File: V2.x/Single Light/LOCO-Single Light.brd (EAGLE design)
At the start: 25.1 x 16.5 mm, 32 parts, among them IC1 Atmega 328-P, IC2 MCP2515, IC3 MIC5219BM5, Q1 8MHz, Q2 16MHz

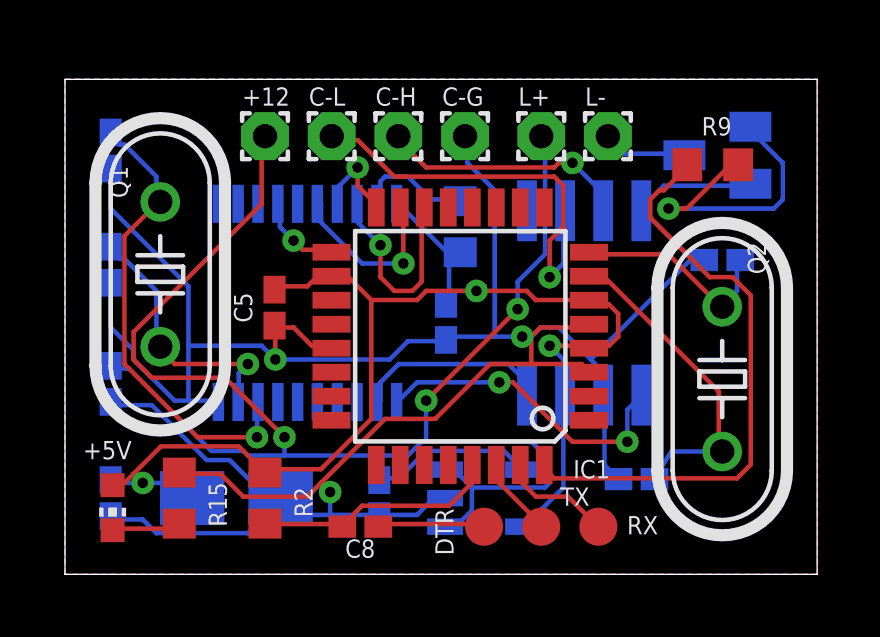
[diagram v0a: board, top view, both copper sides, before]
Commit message: initial
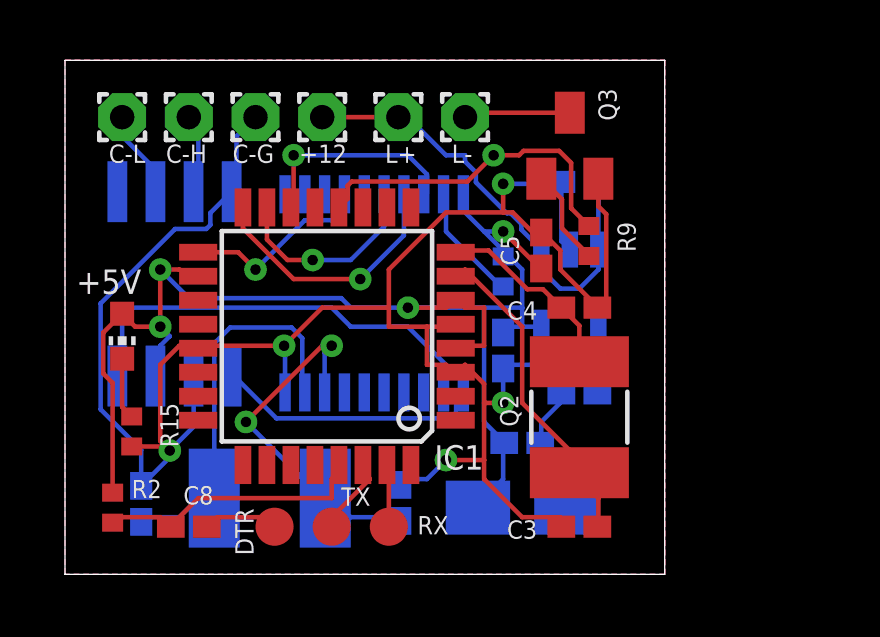
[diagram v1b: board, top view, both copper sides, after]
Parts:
- removed T1: (no value), transistor-neu-to92:SOT23-BEC
- added Q3: BSS123, transistor-small-signal:SOT23
- Q1, Q2: device crystal:HC49/S -> crystal-geyer_V1_0:5.0X3.2_2
- R1, R15, R2, R9: device rcl:R0603 -> rcl:R0402
- moved C11 17.0 mm to (17.1, 13.1), turned to 180 degrees
- moved C2 15.2 mm to (11.2, 2.38), turned to 90 degrees
- moved C15 13.8 mm to (15.2, 4.38), turned to 0 degrees
- moved DA1 13.7 mm to (3.65, 9.68)
- moved C16 9.53 mm to (15.2, 2.22)
- moved C5 9.09 mm to (15.9, 10.8), turned to 270 degrees
- moved Q1 8.31 mm to (6.83, 2.54), flipped to the bottom, turned to 180 degrees
- moved C1 8.03 mm to (2.54, 2.35), turned to 90 degrees
- moved IC3 7.55 mm to (16.8, 9.53), turned to 180 degrees
- moved C7 7.53 mm to (17.1, 6.03), turned to 180 degrees
- moved C-G 7.01 mm to (6.35, 15.2)
- moved C-H 7.01 mm to (4.13, 15.2)
- moved C-L 7.01 mm to (1.91, 15.2)
- moved RX 6.99 mm to (10.8, 1.59)
- moved DTR 6.99 mm to (6.99, 1.59)
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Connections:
- net D2: no longer R9.2
- net D8: now also R9.2
- net GND: now also Q3.2; no longer T1.E
- net LIGHT: now also Q3.3; no longer T1.C
- net N$2: now also Q3.1; no longer T1.B
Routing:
- net +12V: track 50.6 -> 15.6 mm, vias 3 -> 0
- net D2: track 19.7 -> 0.00 mm
- net GND: track 96.6 -> 79.8 mm, vias 3 -> 5
- net D8: track 0.00 -> 11.3 mm, vias 0 -> 1
- net CAN-L: track 14.1 -> 3.03 mm, vias 1 -> 0
- net RXCAN: track 6.55 -> 14.8 mm
- net N$2: track 9.75 -> 3.23 mm, vias 1 -> 0
- net SI: track 3.07 -> 8.74 mm
- net CAN-H: track 8.39 -> 2.82 mm, vias 1 -> 0
- net CAN-OCC1: track 8.75 -> 13.2 mm, vias 1 -> 0
- net SCK: track 2.92 -> 6.44 mm
- net N$1: track 5.46 -> 2.25 mm
- net CAN-OCC2: track 15.6 -> 12.6 mm, vias 1 -> 2
- net RX: track 3.75 -> 2.06 mm
- net VCC: track 46.5 -> 48.2 mm, vias 3 -> 4
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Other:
- board size 25.1 x 16.5 mm -> 20 x 17.1 mm

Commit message: initial
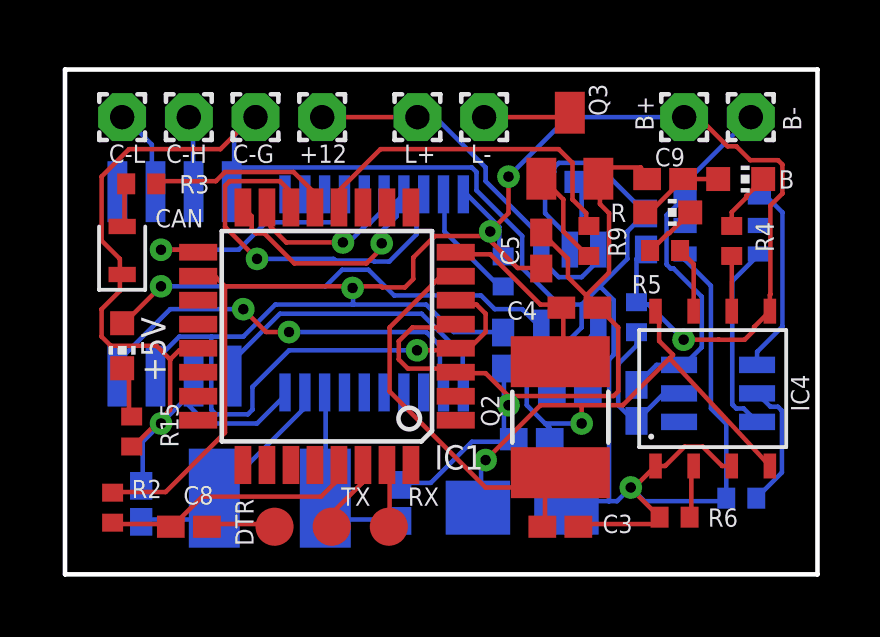
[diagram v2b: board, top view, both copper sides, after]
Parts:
- added B, R: (no value), led:CHIP-LED0603
- added B+, B-: (no value), wirepad:1,6/0,8
- added C10: 0,1µ, rcl:C0402K
- added C12: 10µ, rcl:C0402K
- added C9: 100n, rcl:C0402K
- added CAN: LED1, Opto-Electronic:LEDC1608X39N_B
- added IC4: TP4056, TP4056:SOT23-8
- added IC5: DW01A, DW01a:SOT23-6
- added Q4: FS8205ASOT-23-6L_TCP-L, FS8205A:SOT-23-6L_TCP-L
- added R3: 220R, rcl:R0402
- added R4, R5, R7: 1k, rcl:R0402
- added R6: 1k2, rcl:R0402
- added R8: 100R, rcl:R0402
- R15: value 10k -> 220R
- moved L+ 0.63 mm to (11.7, 15.2)
- moved L- 0.63 mm to (14.0, 15.2)
- moved C11 0.63 mm to (16.5, 13.1)
- moved C3 0.63 mm to (16.5, 1.59), turned to 0 degrees
- moved Q2 0.63 mm to (16.5, 5.24)
- moved C15 0.34 mm to (15.6, 4.51), turned to 180 degrees
- moved +5V 0.32 mm to (1.91, 7.62)
- moved C7 0.32 mm to (16.8, 6.03)
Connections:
- new net +5V: +5V.A, C15.2, C16.+, IC3.5, IC4.4, IC4.8
- new net B-: B-.1, C10.1, IC5.6, Q4.3
- new net N$13: B.A, C9.2, R.A
- new net N$14: IC5.3, Q4.6
- new net N$16: IC5.1, Q4.4
- new net N$17: C10.2, IC5.5, R8.2
- new net N$18: IC5.2, R7.1
- new net N$3: CAN.2, R3.2
- new net N$4: B.C, R4.1
- new net N$5: R.C, R5.1
- new net N$7: IC4.6, R4.2
- new net N$8: IC4.7, R5.2
- new net N$9: IC4.2, R6.2
- net D9: now also R3.1
- net GND: now also C12.1, C9.1, CAN.1, IC4.1, IC4.3, Q4.1, R6.1, R7.2
- net VCC: now also B+.1, C12.2, IC4.5, R8.1; no longer +5V.A, C15.2, C16.+, IC3.5
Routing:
- net GND: track 79.8 -> 125.7 mm, vias 5 -> 3
- net +5V: track 0.00 -> 37.6 mm, vias 0 -> 3
- net VCC: track 48.2 -> 79.9 mm, vias 4 -> 5
- net B-: track 0.00 -> 12.1 mm
- net N$14: track 0.00 -> 6.46 mm
- net N$16: track 0.00 -> 6.41 mm
- net D9: track 0.00 -> 6.26 mm
- net CAN-OCC2: track 12.6 -> 6.39 mm, vias 2 -> 0
- net CS: track 7.20 -> 13.0 mm
- net CAN-OCC1: track 13.2 -> 7.54 mm
- net N$17: track 0.00 -> 5.43 mm
- net N$18: track 0.00 -> 4.34 mm
- net N$10: track 10.8 -> 14.3 mm
- net N$13: track 0.00 -> 2.89 mm
- net N$8: track 0.00 -> 2.21 mm
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- removed copper zone on layer 1, net GND
- removed copper zone on layer 16, net GND
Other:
- board size 20 x 17.1 mm -> 25.1 x 16.8 mm
- board text added: "LOCO-Single"
- board text added: "V2.1-s"
- board text removed: "LOCO-Single-Light"
- board text removed: "V2.0-s"
